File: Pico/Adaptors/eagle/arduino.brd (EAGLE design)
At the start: 57.5 x 53.3 mm, 3 parts

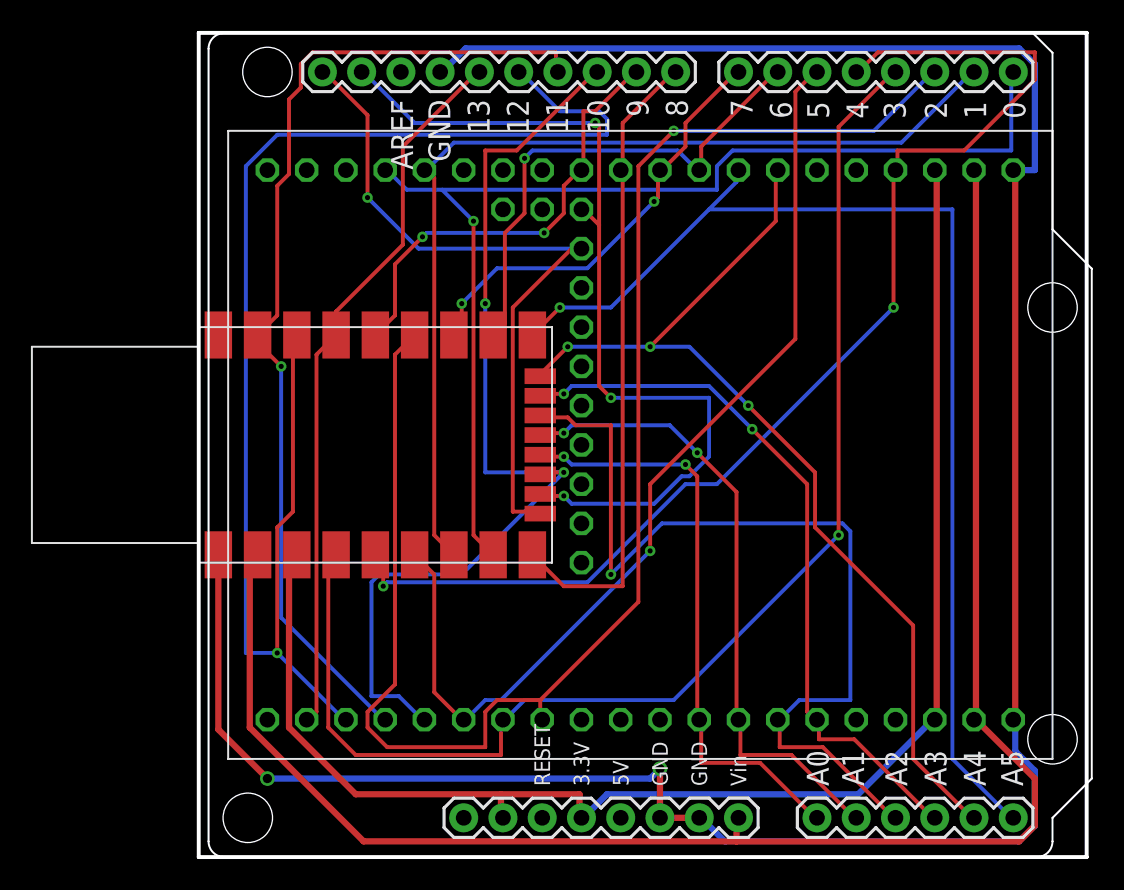
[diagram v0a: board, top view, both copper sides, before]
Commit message: tweaking
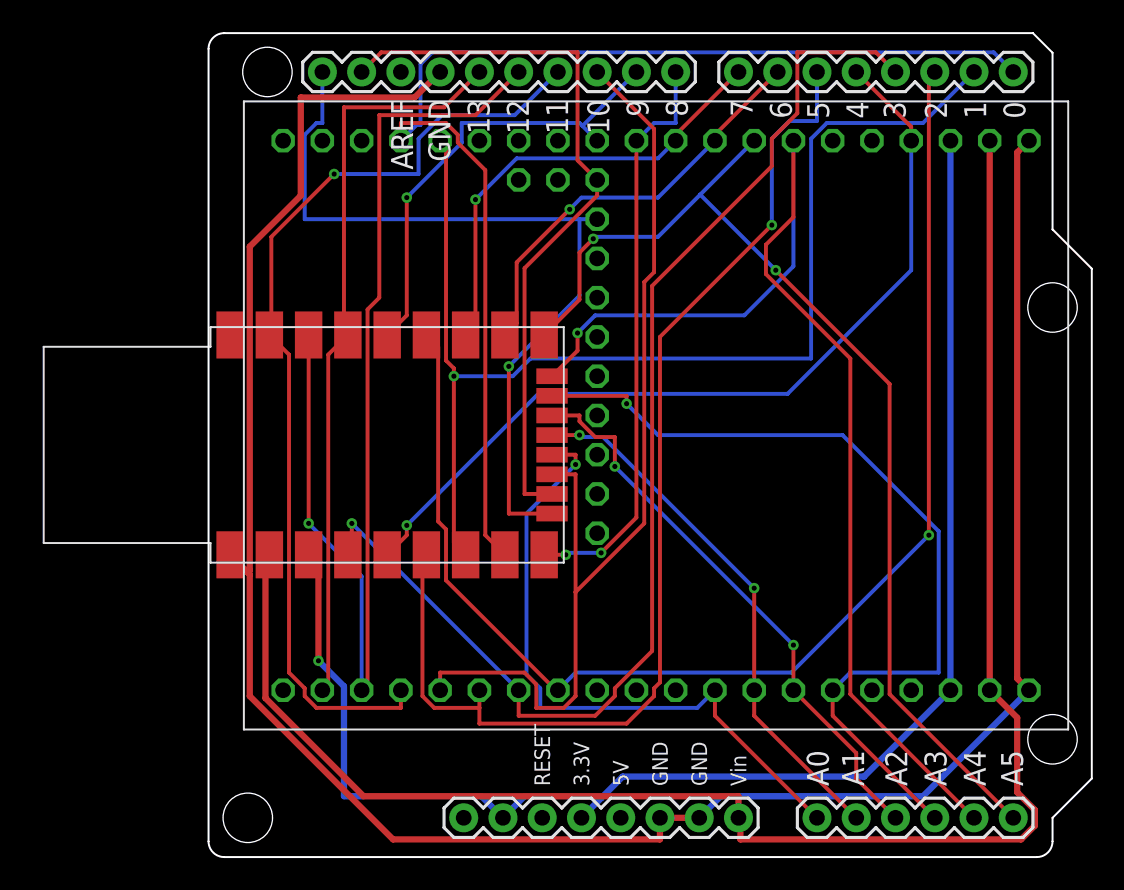
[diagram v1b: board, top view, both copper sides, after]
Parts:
- moved U$3 2.16 mm to (29.6, 29.8)
- moved U$1 0.76 mm to (16.0, 26.7)
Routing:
- net A2: track 59.1 -> 37.0 mm, vias 1 -> 2
- net D4: track 77.8 -> 56.2 mm, vias 2 -> 1
- net D12: track 93.1 -> 72.3 mm
- net D2: track 101.2 -> 84.9 mm
- net GND: track 161.1 -> 146.8 mm, vias 2 -> 0
- net A4: track 63.6 -> 77.5 mm, vias 3 -> 1
- net D1: track 63.9 -> 77.6 mm, vias 0 -> 1
- net SDA: track 58.9 -> 47.3 mm, vias 3 -> 0
- net A3: track 46.8 -> 56.4 mm, vias 2 -> 1
- net D5: track 64.2 -> 73.2 mm
- net SCL: track 45.8 -> 52.9 mm
- net A1: track 41.3 -> 34.8 mm
- net A5: track 75.0 -> 69.3 mm, vias 1 -> 2
- net D6: track 32.9 -> 27.2 mm
- net D0: track 73.2 -> 78.4 mm, vias 1 -> 0
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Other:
- board size 57.5 x 53.3 mm -> 57.1 x 53.3 mm
